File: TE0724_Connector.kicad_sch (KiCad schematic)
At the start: 1 part, among them J1 SS5-80-3.50-X-D-K-XX

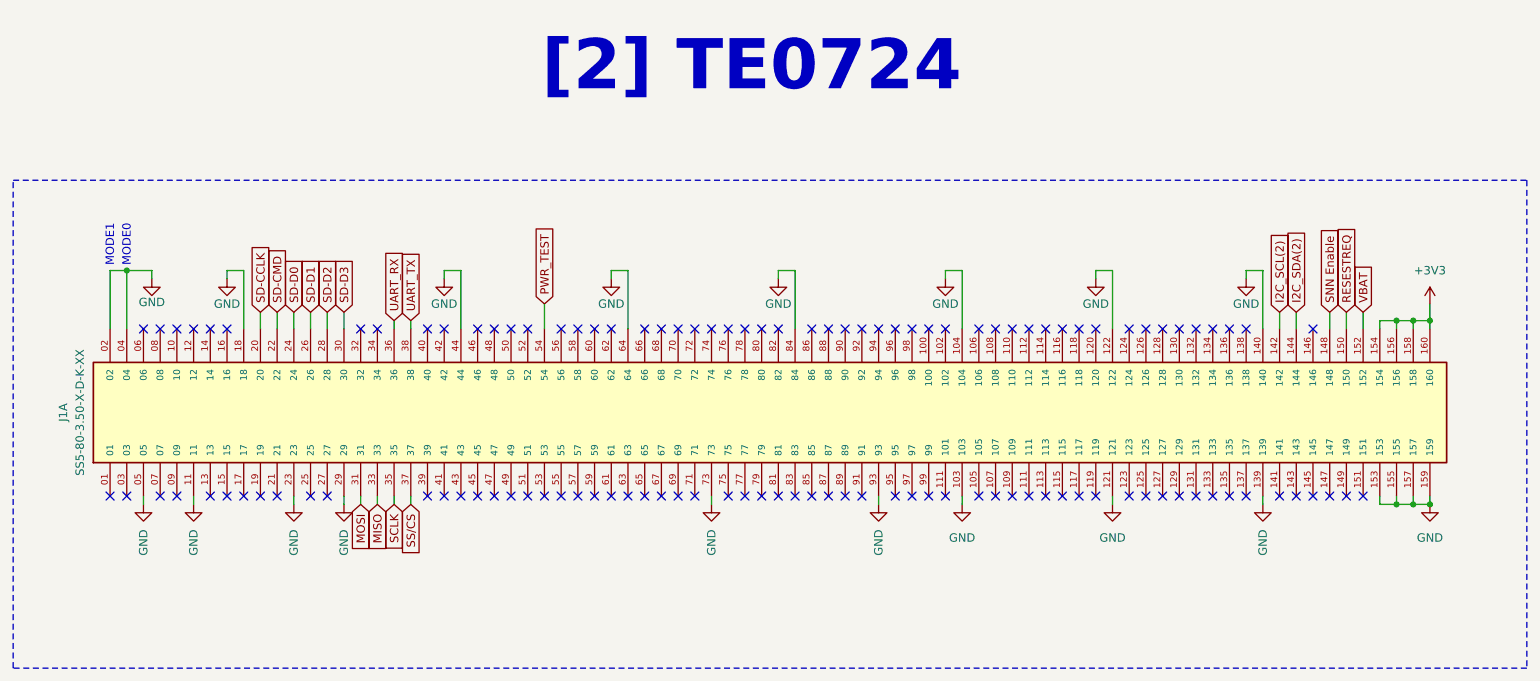
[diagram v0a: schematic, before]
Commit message: fixed 3D models
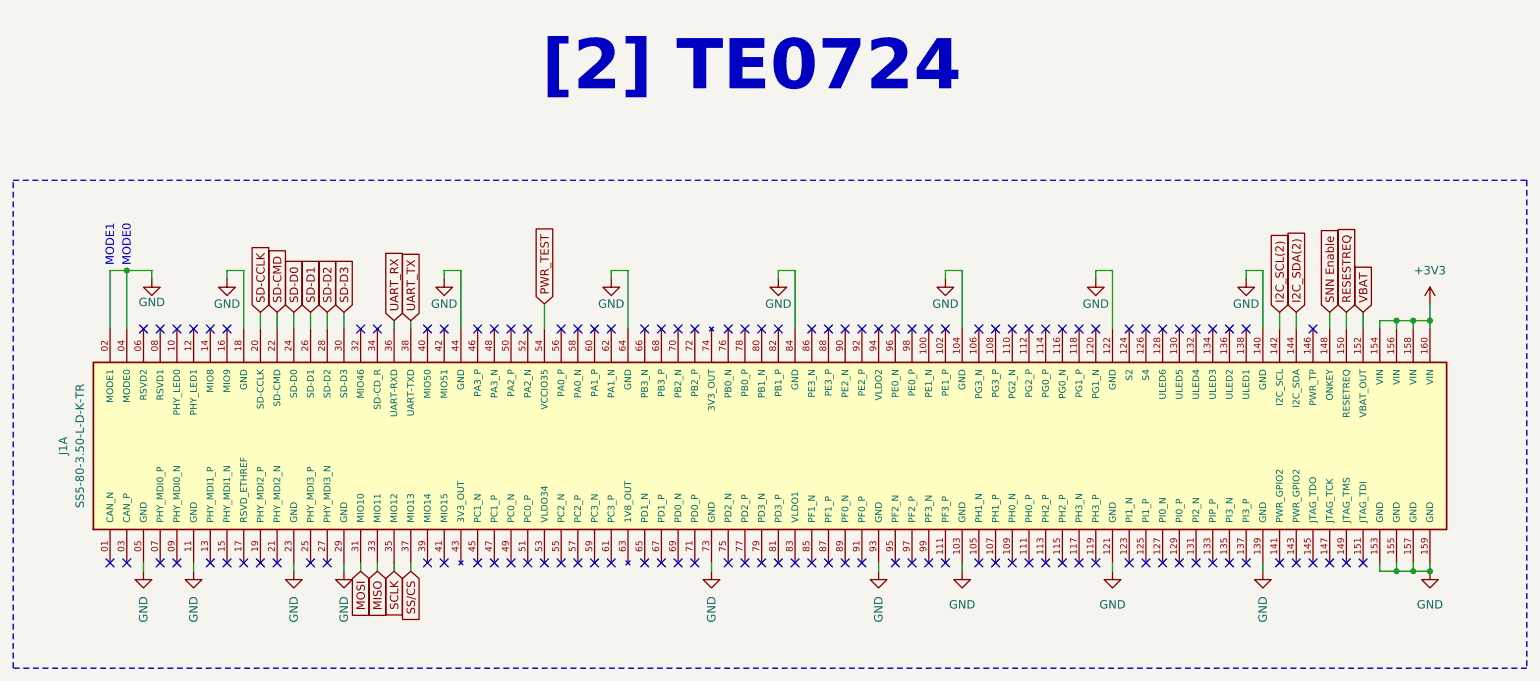
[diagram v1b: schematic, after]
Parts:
- J1: value SS5-80-3.50-X-D-K-XX -> SS5-80-3.50-L-D-K-TR
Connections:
- no-connect marks 116 -> 113
